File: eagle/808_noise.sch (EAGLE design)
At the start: 20 parts, among them IC1 TL072P, Q1 2N3904, U24 µPC4558C

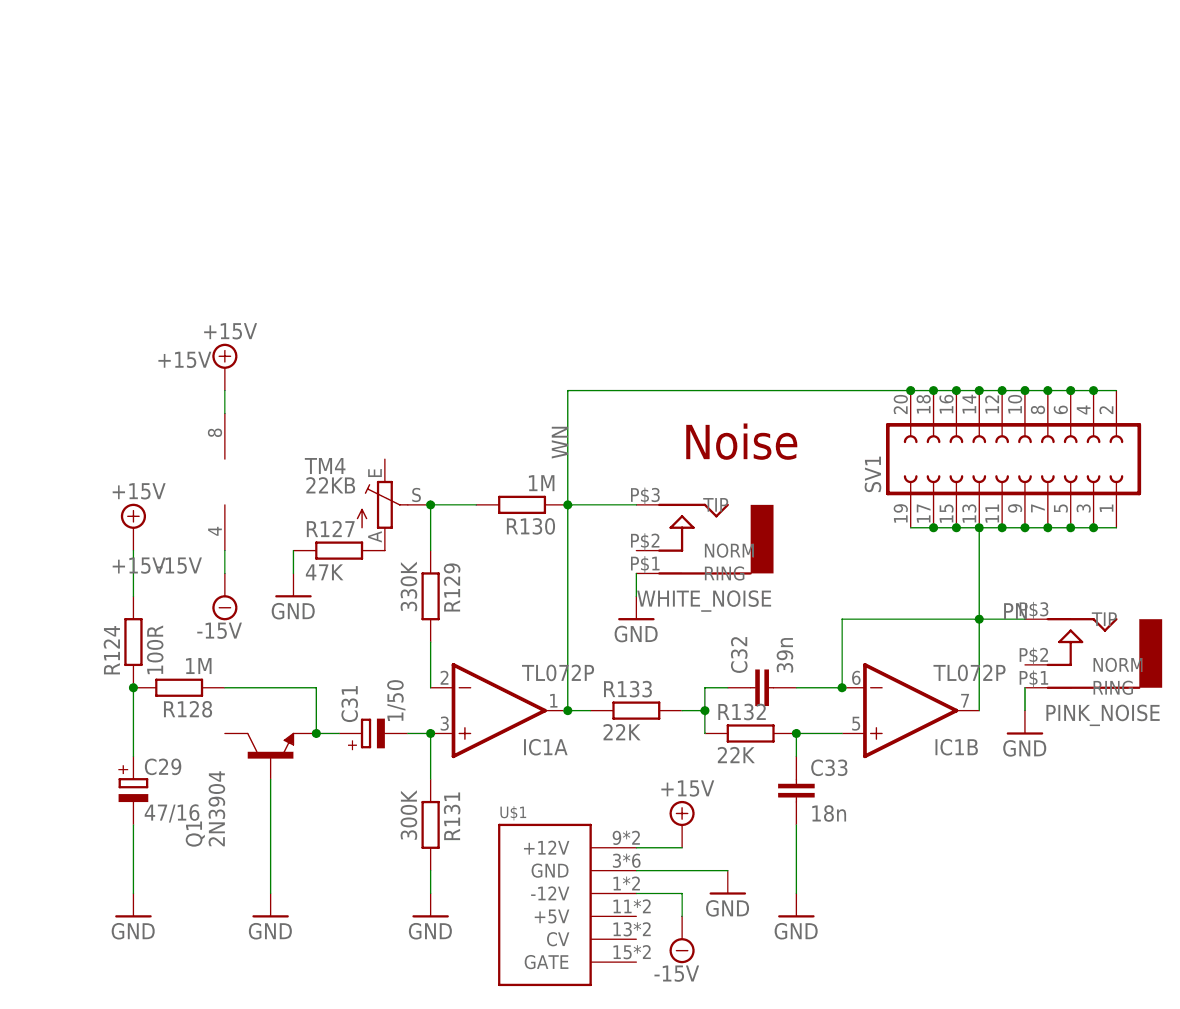
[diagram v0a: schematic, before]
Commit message: routed
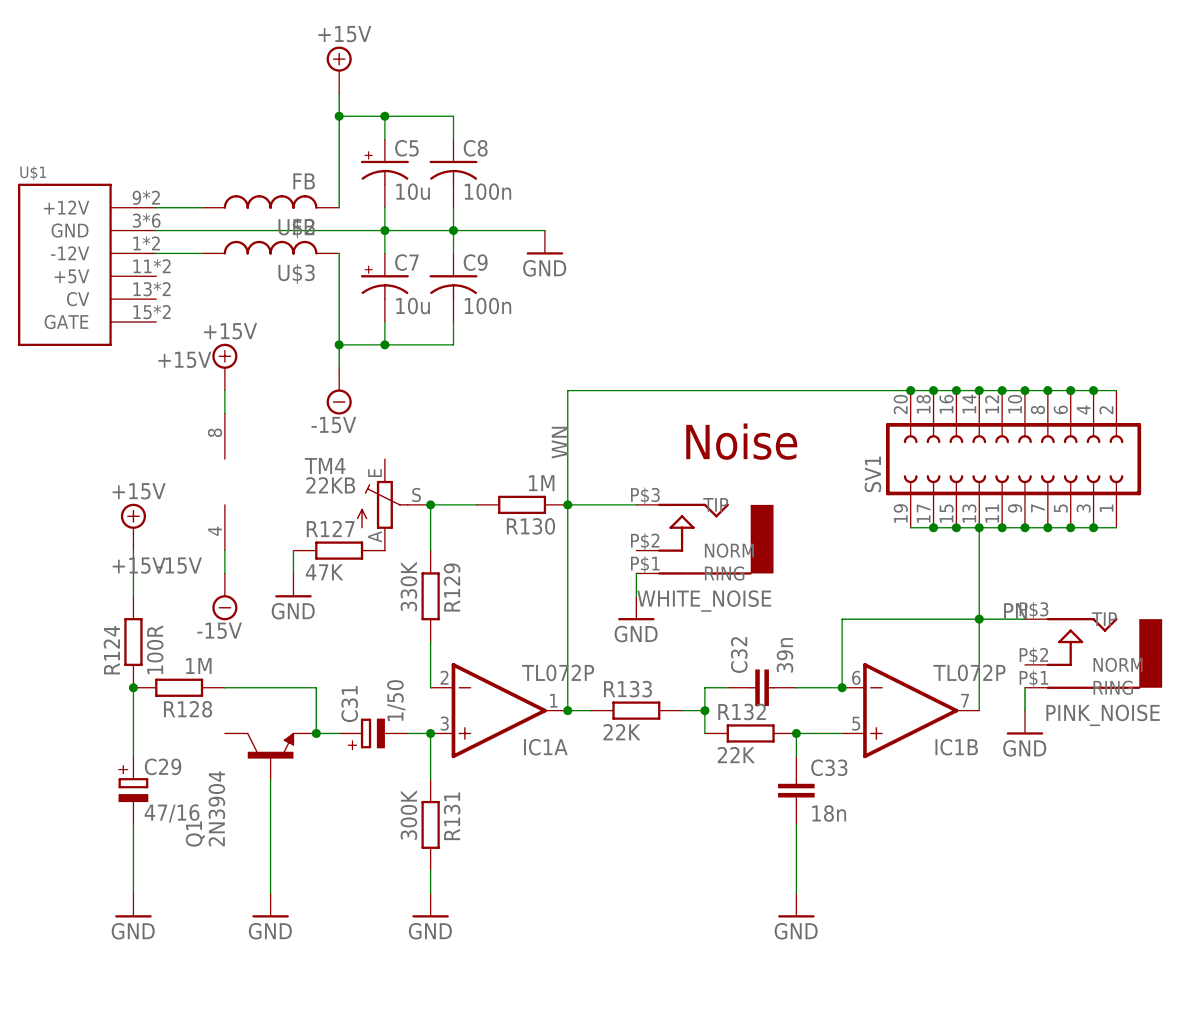
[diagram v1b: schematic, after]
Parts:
- removed U24: µPC4558C, TR808clone:µPC4558C
- added C5, C7: 10u, rcl:CPOL-USB45181A
- added C8, C9: 100n, rcl:C-US050-024X044
- added U$2, U$3: FB, adafruit:FB
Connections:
- new net N$11: U$1.+12V, U$2.1
- new net N$18: U$1.-12V, U$3.1
- net +15V: now also C5.+, C8.1, IC1P.V+, U$2.2; no longer U$1.+12V, U24G$3.V+
- net -15V: now also C7.-, C9.2, IC1P.V-, U$3.2; no longer U$1.-12V, U24G$3.V-
- net GND: now also C5.-, C7.+, C8.2, C9.1
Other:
- moved on the sheet: U$1
